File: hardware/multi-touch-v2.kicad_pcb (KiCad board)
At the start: 2 copper layers, 25 x 30 mm, 31 parts, among them P1 CON-SENSOR2, P2 DEBUG, P3 BOOT, P4 CONN_01X12, U1 MPR121Q, U2 XMC1100, U3 DRILL, U4 DRILL, U5 DRILL, U6 DRILL

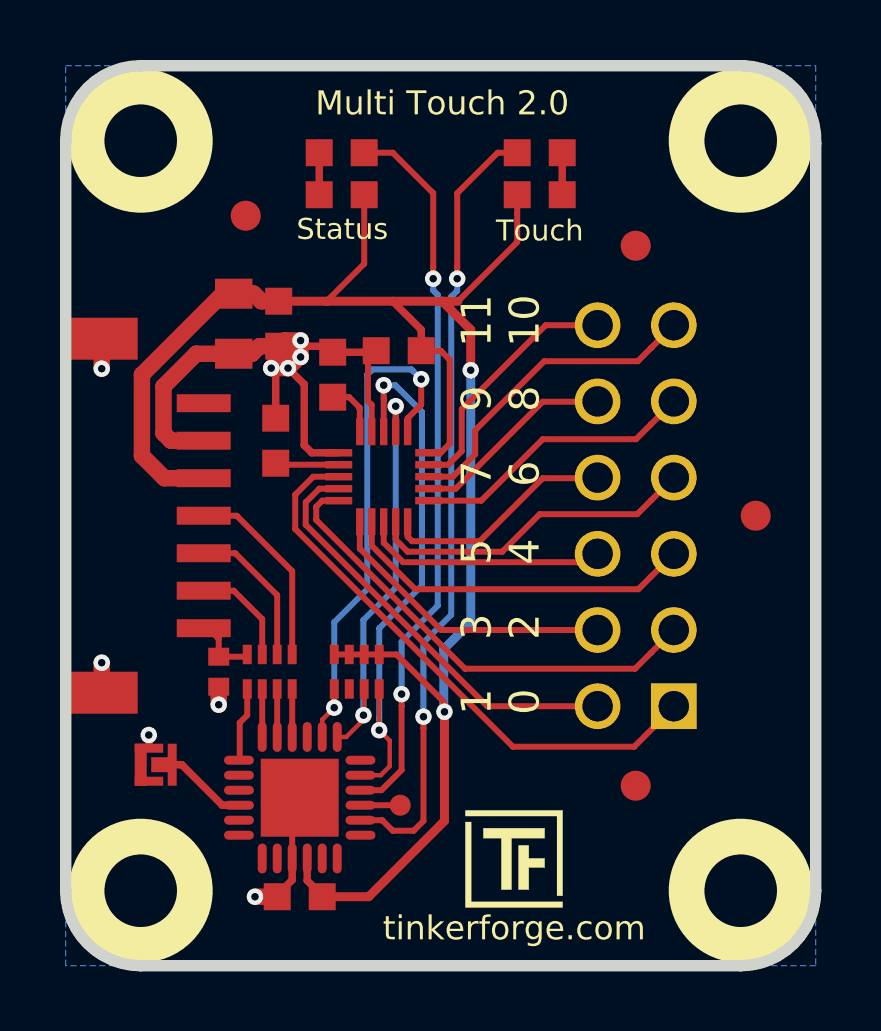
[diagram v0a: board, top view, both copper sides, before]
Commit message: drc
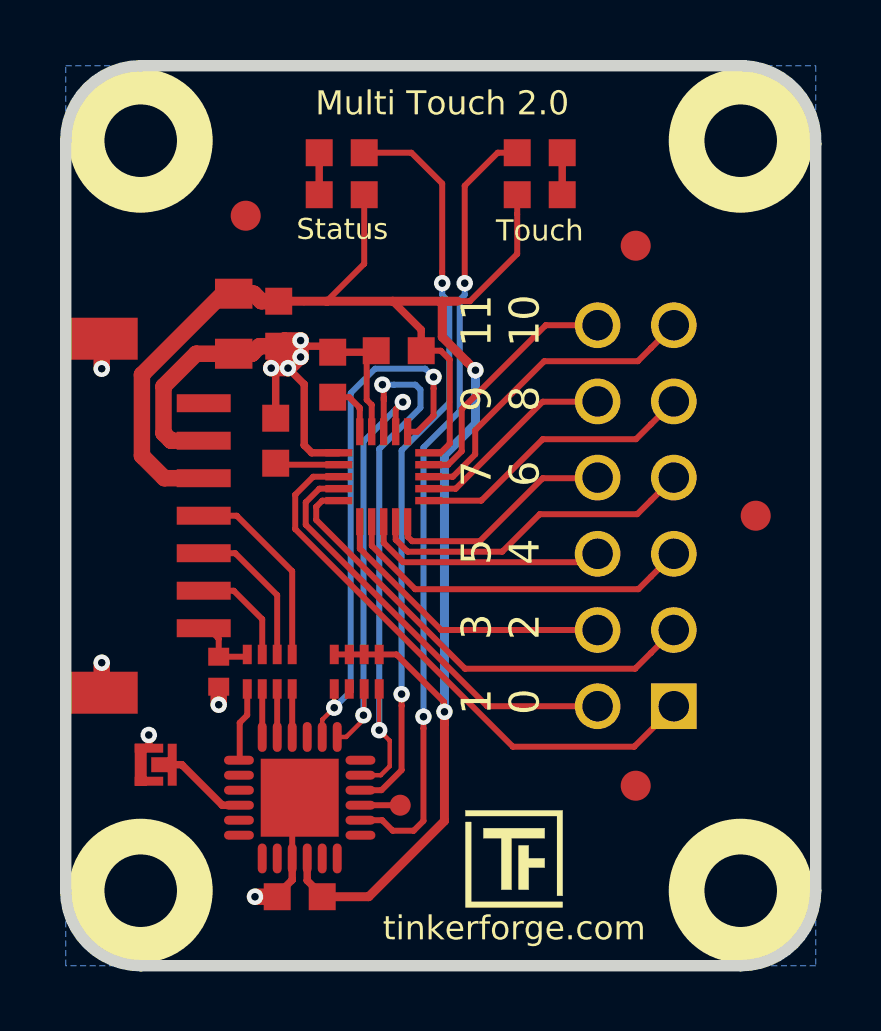
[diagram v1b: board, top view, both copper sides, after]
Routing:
- net INT: track 17.3 -> 18.1 mm
- net Net-(R5-Pad1): track 24.3 -> 25.0 mm
- net SCL: track 13.5 -> 14.0 mm
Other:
- net class Default: clearance 0.15 -> 0.149
- rule trace_clearance: 0.15 -> 0.149
